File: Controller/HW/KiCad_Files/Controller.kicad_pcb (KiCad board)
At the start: 4 copper layers, 70 x 70 mm, 86 parts, among them J1 USB, J2 JTAG, J3 Speaker, J4 Driver, J5 Groove, J6 QWIIC, Q1 MMBT3904, Q2 MMBT3904, Q3 MMBT3904, Q4 NX138AK, Q5 NX138AK, SW1 ESP Config, SW2 Reset, SW3 Gain, U1 AP1117-33, U2 USBLC6-2SC6, U3 CP2102N-Axx-xQFN28, U4 ESP32-S3-WROOM-1, U5 MAX98357A

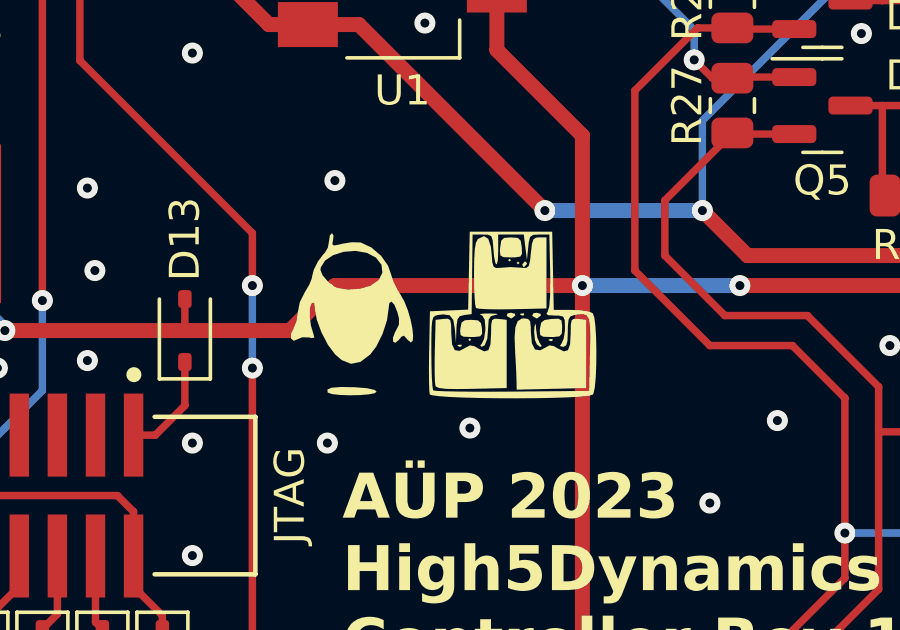
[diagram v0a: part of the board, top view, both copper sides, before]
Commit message: BOM update
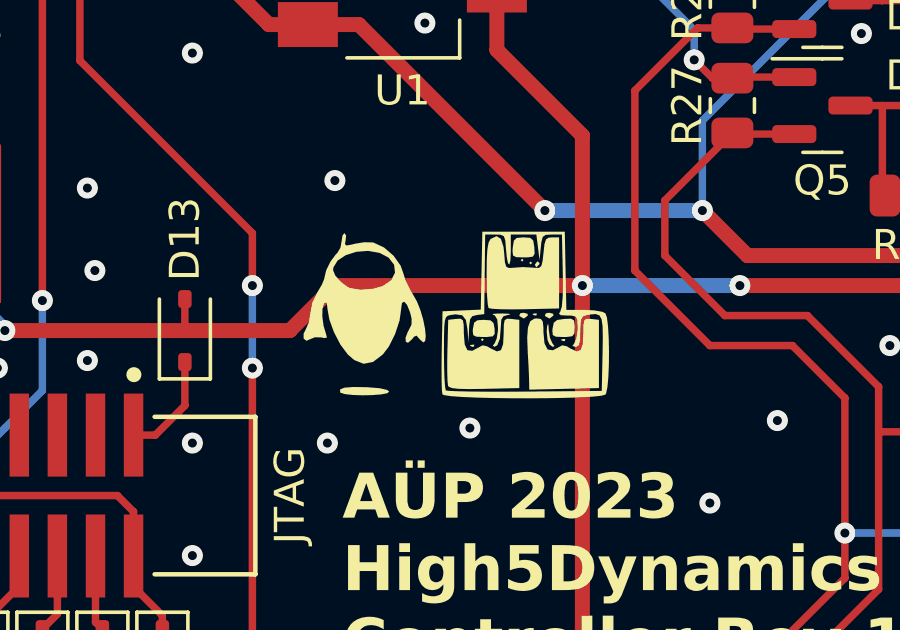
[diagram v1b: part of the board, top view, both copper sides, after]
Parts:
- moved G*** 0.42 mm to (153.5, 81.9)
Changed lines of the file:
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@@
   )
   (footprint "LOGO" (layer "F.Cu")
-    (at 153.08 81.905)
+    (at 153.5 81.905)
     (attr board_only exclude_from_pos_files exclude_from_bom)
     (fp_text reference "G***" (at 0 0) (layer "F.SilkS") hide
